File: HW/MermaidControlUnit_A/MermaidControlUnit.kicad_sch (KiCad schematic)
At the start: 0 parts

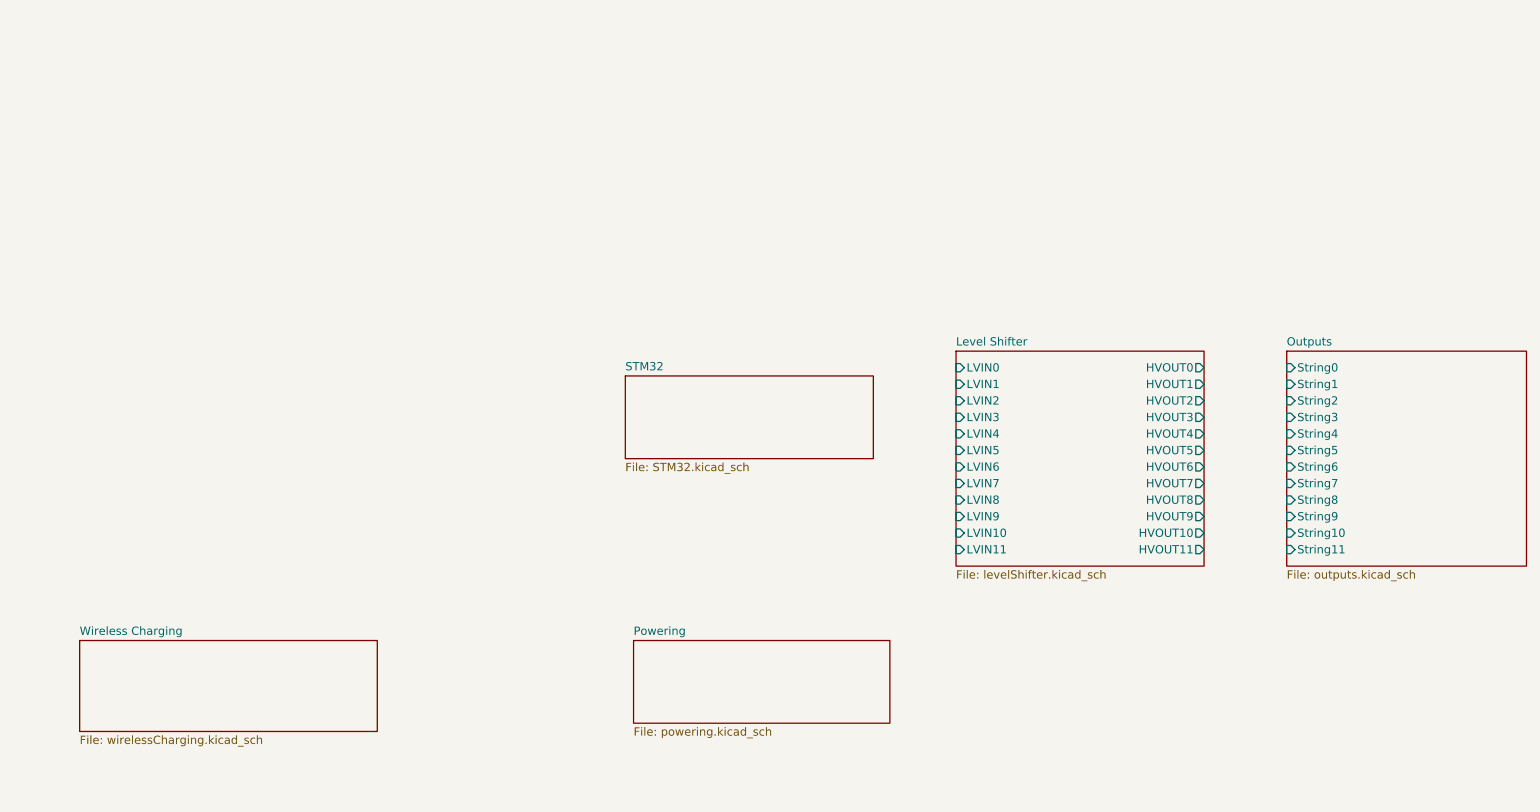
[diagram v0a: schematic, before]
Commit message: HW design progress
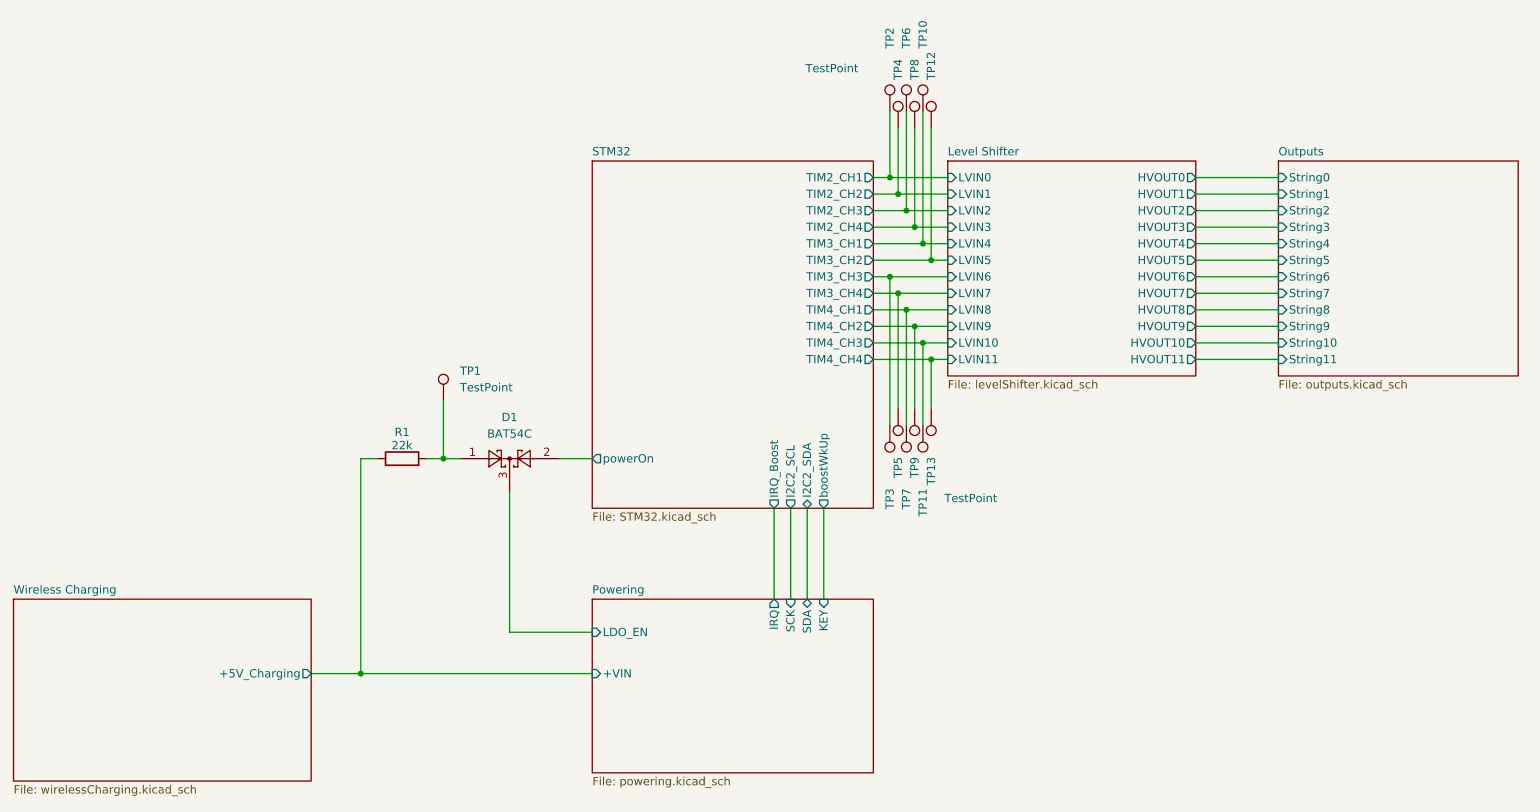
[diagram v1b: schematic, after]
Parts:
- added D1: BAT54C, Package_TO_SOT_SMD:SOT-23, symbol Diode:BAT54C
- added R1: 22k, Resistor_SMD:R_0603_1608Metric, symbol Device:R
- added TP1, TP10, TP11, TP12, TP13, TP2, TP3, TP4, TP5, TP6, TP7, TP8, TP9: TestPoint, TestPoint:TestPoint_Pad_D2.0mm, symbol Connector:TestPoint
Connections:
- net Level Shifter/LVIN0: now also TP2.1
- net Level Shifter/LVIN1: now also TP4.1
- net Level Shifter/LVIN10: now also TP11.1
- net Level Shifter/LVIN11: now also TP13.1
- net Level Shifter/LVIN2: now also TP6.1
- net Level Shifter/LVIN3: now also TP8.1
- net Level Shifter/LVIN4: now also TP10.1
- net Level Shifter/LVIN5: now also TP12.1
- net Level Shifter/LVIN6: now also TP3.1
- net Level Shifter/LVIN7: now also TP5.1
- net Level Shifter/LVIN8: now also TP7.1
- net Level Shifter/LVIN9: now also TP9.1
- new net: D1.1, R1.2, TP1.1
- new net Powering/+VIN: R1.1
- new net Powering/LDO_EN: D1.3
- new net STM32/powerOn: D1.2
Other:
- sheet Powering ports: added +VIN, IRQ, KEY, LDO_EN, SCK, SDA; removed none
- sheet STM32 ports: added I2C2_SCL, I2C2_SDA, IRQ_Boost, TIM2_CH1, TIM2_CH2, TIM2_CH3, TIM2_CH4, TIM3_CH1, TIM3_CH2, TIM3_CH3, TIM3_CH4, TIM4_CH1, TIM4_CH2, TIM4_CH3, TIM4_CH4, boostWkUp, powerOn; removed none
- sheet Wireless Charging ports: added +5V_Charging; removed none

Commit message: hw progress
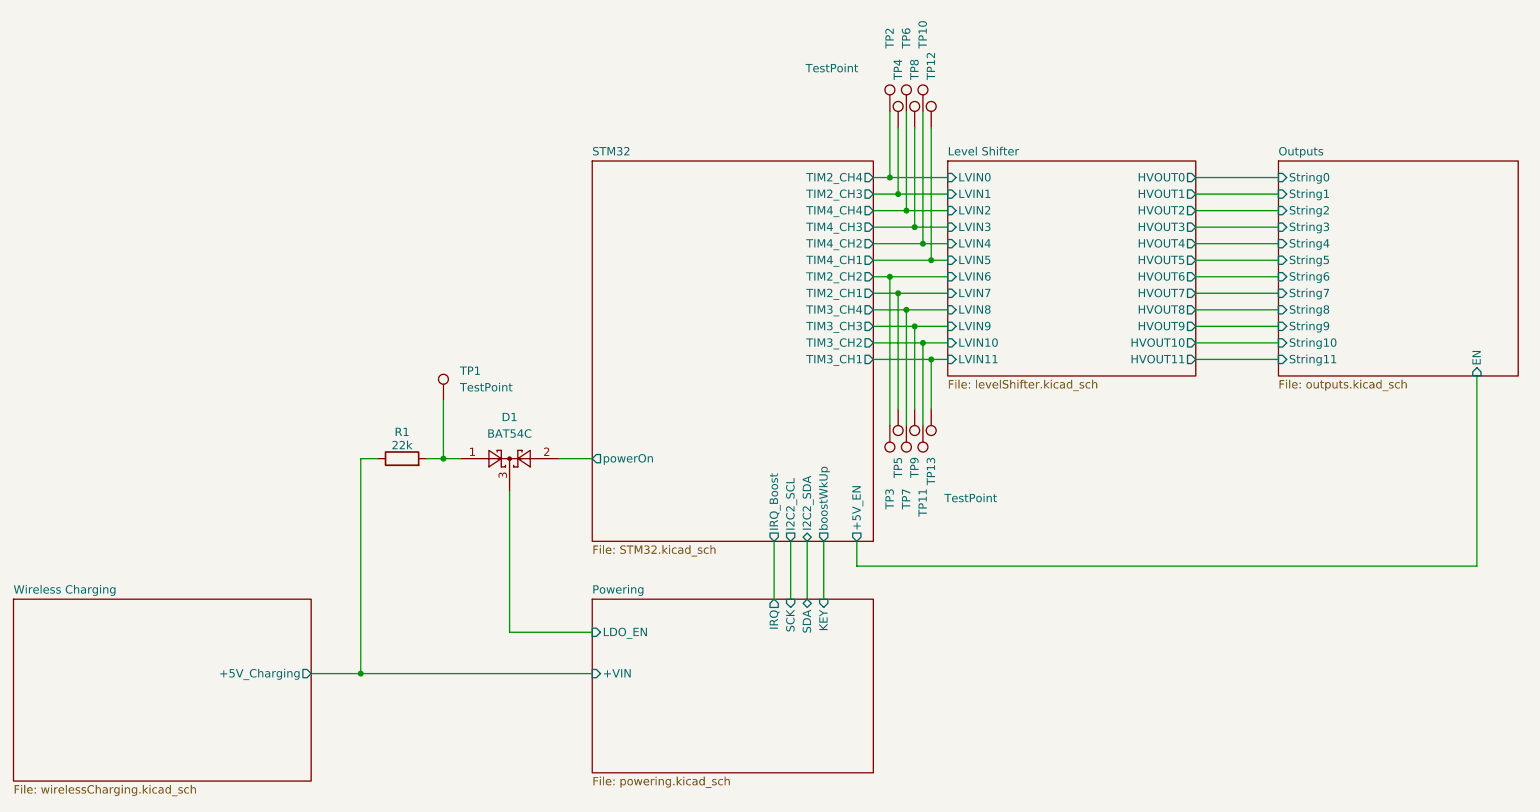
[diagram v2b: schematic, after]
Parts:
- TP1, TP10, TP11, TP12, TP13, TP2, TP3, TP4, TP5, TP6, TP7, TP8, TP9: footprint TestPoint:TestPoint_Pad_D2.0mm -> TestPoint:TestPoint_Pad_D1.5mm
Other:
- sheet Outputs ports: added EN; removed none
- sheet STM32 ports: added +5V_EN; removed none
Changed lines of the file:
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@@
+	(wire
+		(pts
+			(xy 161.29 105.41) (xy 256.54 105.41)
+		)
+		(stroke
+			(width 0)
+			(type default)
+		)
+	)
 	(wire
 		(pts
@@
 	(wire
 		(pts
+			(xy 153.67 101.6) (xy 153.67 110.49)
+		)
+		(stroke
+			(width 0)
+			(type default)
+		)
+	)
+	(wire
+		(pts
 			(xy 172.72 73.66) (xy 175.26 73.66)
 		)
@@
 	(wire
 		(pts
+			(xy 161.29 101.6) (xy 161.29 105.41)
+		)
+		(stroke
+			(width 0)
+			(type default)
+		)
+	)
+	(wire
+		(pts
 			(xy 166.37 60.96) (xy 166.37 83.82)
 		)
@@
 	(wire
 		(pts
+			(xy 148.59 101.6) (xy 148.59 110.49)
+		)
+		(stroke
+			(width 0)
+			(type default)
+		)
+	)
+	(wire
+		(pts
 			(xy 163.83 53.34) (xy 170.18 53.34)
 		)
@@
 	(wire
 		(pts
-			(xy 148.59 96.52) (xy 148.59 110.49)
-		)
-		(stroke
-			(width 0)
-			(type default)
-		)
-	)
-	(wire
-		(pts
 			(xy 213.36 63.5) (xy 226.06 63.5)
 		)
@@
 	(wire
 		(pts
-			(xy 153.67 96.52) (xy 153.67 110.49)
+			(xy 156.21 101.6) (xy 156.21 110.49)
 		)
 		(stroke
@@
 	(wire
 		(pts
-			(xy 156.21 96.52) (xy 156.21 110.49)
-		)
-		(stroke
-			(width 0)
-			(type default)
-		)
-	)
-	(wire
-		(pts
 			(xy 167.64 63.5) (xy 175.26 63.5)
 		)
@@
 	(wire
 		(pts
+			(xy 256.54 105.41) (xy 256.54 76.2)
+		)
+		(stroke
+			(width 0)
+			(type default)
+		)
+	)
+	(wire
+		(pts
 			(xy 168.91 35.56) (xy 168.91 50.8)
 		)
@@
 	(wire
 		(pts
-			(xy 151.13 96.52) (xy 151.13 110.49)
+			(xy 151.13 101.6) (xy 151.13 110.49)
 		)
 		(stroke
@@
 			)
 		)
-		(property "Footprint" "TestPoint:TestPoint_Pad_D2.0mm"
+		(property "Footprint" "TestPoint:TestPoint_Pad_D1.5mm"
 			(at 171.45 35.56 0)
 			(effects
@@
 			)
 		)
-		(property "Footprint" "TestPoint:TestPoint_Pad_D2.0mm"
+		(property "Footprint" "TestPoint:TestPoint_Pad_D1.5mm"
 			(at 177.8 81.28 0)
 			(effects
@@
 			)
 		)
-		(property "Footprint" "TestPoint:TestPoint_Pad_D2.0mm"
+		(property "Footprint" "TestPoint:TestPoint_Pad_D1.5mm"
 			(at 172.72 81.28 0)
 			(effects
@@
 			)
 		)
-		(property "Footprint" "TestPoint:TestPoint_Pad_D2.0mm"
+		(property "Footprint" "TestPoint:TestPoint_Pad_D1.5mm"
 			(at 172.72 38.1 0)
 			(effects
@@
 			)
 		)
-		(property "Footprint" "TestPoint:TestPoint_Pad_D2.0mm"
+		(property "Footprint" "TestPoint:TestPoint_Pad_D1.5mm"
 			(at 173.99 35.56 0)
 			(effects
@@
 			)
 		)
-		(property "Footprint" "TestPoint:TestPoint_Pad_D2.0mm"
+		(property "Footprint" "TestPoint:TestPoint_Pad_D1.5mm"
 			(at 175.26 81.28 0)
 			(effects
@@
 			)
 		)
-		(property "Footprint" "TestPoint:TestPoint_Pad_D2.0mm"
+		(property "Footprint" "TestPoint:TestPoint_Pad_D1.5mm"
 			(at 177.8 38.1 0)
 			(effects
@@
 			)
 		)
-		(property "Footprint" "TestPoint:TestPoint_Pad_D2.0mm"
+		(property "Footprint" "TestPoint:TestPoint_Pad_D1.5mm"
 			(at 171.45 83.82 0)
 			(effects
@@
 			)
 		)
-		(property "Footprint" "TestPoint:TestPoint_Pad_D2.0mm"
+		(property "Footprint" "TestPoint:TestPoint_Pad_D1.5mm"
 			(at 175.26 38.1 0)
 			(effects
@@
 			)
 		)
-		(property "Footprint" "TestPoint:TestPoint_Pad_D2.0mm"
+		(property "Footprint" "TestPoint:TestPoint_Pad_D1.5mm"
 			(at 176.53 83.82 0)
 			(effects
@@
 			)
 		)
-		(property "Footprint" "TestPoint:TestPoint_Pad_D2.0mm"
+		(property "Footprint" "TestPoint:TestPoint_Pad_D1.5mm"
 			(at 176.53 35.56 0)
 			(effects
@@
 			)
 		)
-		(property "Footprint" "TestPoint:TestPoint_Pad_D2.0mm"
+		(property "Footprint" "TestPoint:TestPoint_Pad_D1.5mm"
 			(at 102.87 80.01 0)
 			(effects
@@
 			)
 		)
-		(property "Footprint" "TestPoint:TestPoint_Pad_D2.0mm"
+		(property "Footprint" "TestPoint:TestPoint_Pad_D1.5mm"
 			(at 173.99 83.82 0)
 			(effects
@@
 	(sheet
 		(at 120.65 43.18)
-		(size 43.18 53.34)
+		(size 43.18 58.42)
 		(fields_autoplaced yes)
 		(stroke
@@
 		)
 		(property "Sheetfile" "STM32.kicad_sch"
-			(at 120.65 97.1046 0)
+			(at 120.65 102.1846 0)
 			(effects
 				(font
@@
 		)
 		(pin "TIM4_CH3" output
-			(at 163.83 71.12 0)
+			(at 163.83 53.34 0)
 			(effects
 				(font
@@
 		)
 		(pin "TIM4_CH4" output
-			(at 163.83 73.66 0)
+			(at 163.83 50.8 0)
 			(effects
 				(font
@@
 		)
 		(pin "I2C2_SCL" output
-			(at 151.13 96.52 270)
+			(at 151.13 101.6 270)
 			(effects
 				(font
@@
 		)
 		(pin "I2C2_SDA" bidirectional
-			(at 153.67 96.52 270)
+			(at 153.67 101.6 270)
 			(effects
 				(font
@@
 		)
 		(pin "boostWkUp" output
-			(at 156.21 96.52 270)
+			(at 156.21 101.6 270)
 			(effects
 				(font
@@
 		)
 		(pin "TIM4_CH1" output
+			(at 163.83 58.42 0)
+			(effects
+				(font
+					(size 1.27 1.27)
+				)
+				(justify right)
+			)
+		)
+		(pin "TIM3_CH4" output
 			(at 163.83 66.04 0)
 			(effects
@@
 			)
 		)
-		(pin "TIM3_CH4" output
+		(pin "TIM3_CH3" output
+			(at 163.83 68.58 0)
+			(effects
+				(font
+					(size 1.27 1.27)
+				)
+				(justify right)
+			)
+		)
+		(pin "TIM2_CH2" output
+			(at 163.83 60.96 0)
+			(effects
+				(font
+					(size 1.27 1.27)
+				)
+				(justify right)
+			)
+		)
+		(pin "TIM4_CH2" output
+			(at 163.83 55.88 0)
+			(effects
+				(font
+					(size 1.27 1.27)
+				)
+				(justify right)
+			)
+		)
+		(pin "IRQ_Boost" output
+			(at 148.59 101.6 270)
+			(effects
+				(font
+					(size 1.27 1.27)
+				)
+				(justify left)
+			)
+		)
+		(pin "TIM2_CH4" output
+			(at 163.83 45.72 0)
+			(effects
+				(font
+					(size 1.27 1.27)
+				)
+				(justify right)
+			)
+		)
+		(pin "TIM2_CH3" output
+			(at 163.83 48.26 0)
+			(effects
+				(font
+					(size 1.27 1.27)
+				)
+				(justify right)
+			)
+		)
+		(pin "TIM3_CH1" output
+			(at 163.83 73.66 0)
+			(effects
+				(font
+					(size 1.27 1.27)
+				)
+				(justify right)
+			)
+		)
+		(pin "TIM3_CH2" output
+			(at 163.83 71.12 0)
+			(effects
+				(font
+					(size 1.27 1.27)
+				)
+				(justify right)
+			)
+		)
+		(pin "TIM2_CH1" output
 			(at 163.83 63.5 0)
 			(effects
@@
 			)
 		)
-		(pin "TIM3_CH3" output
-			(at 163.83 60.96 0)
-			(effects
-				(font
-					(size 1.27 1.27)
-				)
-				(justify right)
-			)
-		)
-		(pin "TIM2_CH2" output
-			(at 163.83 48.26 0)
-			(effects
-				(font
-					(size 1.27 1.27)
-				)
-				(justify right)
-			)
-		)
-		(pin "TIM4_CH2" output
-			(at 163.83 68.58 0)
-			(effects
-				(font
-					(size 1.27 1.27)
-				)
-				(justify right)
-			)
-		)
-		(pin "IRQ_Boost" output
-			(at 148.59 96.52 270)
-			(effects
-				(font
-					(size 1.27 1.27)
-				)
-				(justify left)
-			)
-		)
-		(pin "TIM2_CH4" output
-			(at 163.83 53.34 0)
-			(effects
-				(font
-					(size 1.27 1.27)
-				)
-				(justify right)
-			)
-		)
-		(pin "TIM2_CH3" output
-			(at 163.83 50.8 0)
-			(effects
-				(font
-					(size 1.27 1.27)
-				)
-				(justify right)
-			)
-		)
-		(pin "TIM3_CH1" output
-			(at 163.83 55.88 0)
-			(effects
-				(font
-					(size 1.27 1.27)
-				)
-				(justify right)
-			)
-		)
-		(pin "TIM3_CH2" output
-			(at 163.83 58.42 0)
-			(effects
-				(font
-					(size 1.27 1.27)
-				)
-				(justify right)
-			)
-		)
-		(pin "TIM2_CH1" output
-			(at 163.83 45.72 0)
-			(effects
-				(font
-					(size 1.27 1.27)
-				)
-				(justify right)
+		(pin "+5V_EN" output
+			(at 161.29 101.6 270)
+			(effects
+				(font
+					(size 1.27 1.27)
+				)
+				(justify left)
 			)
 		)
@@
 			(effects
 				(font
+					(size 1.27 1.27)
+				)
+				(justify left)
+			)
+		)
+		(pin "EN" input
+			(at 256.54 76.2 270)
+			(effects
+				(font

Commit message: production rev A
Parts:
- D1: Part Number (none) -> BAT54CLT1G
- R1: Part Number (none) -> RC0603FR-0722KL
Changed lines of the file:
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@@
+			)
+		)
+		(property "Part Number" "RC0603FR-0722KL"
+			(at 91.44 88.9 0)
+			(effects
+				(font
+					(size 1.27 1.27)
+				)
+				(hide yes)
 			)
 		)
@@
 			(at 107.95 88.9 0)
 			(effects
+				(font
+					(size 1.27 1.27)
+				)
+				(hide yes)
+			)
+		)
+		(property "Part Number" "BAT54CLT1G"
+			(at 107.95 88.9 0)
+			(effects
